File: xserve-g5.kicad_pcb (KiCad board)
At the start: 2 copper layers, 100 x 50 mm, 4 parts, among them J1 SATA_Backplane_PWR, J2 FAN_LEFT, J3 FAN_RIGHT, J4 PWR

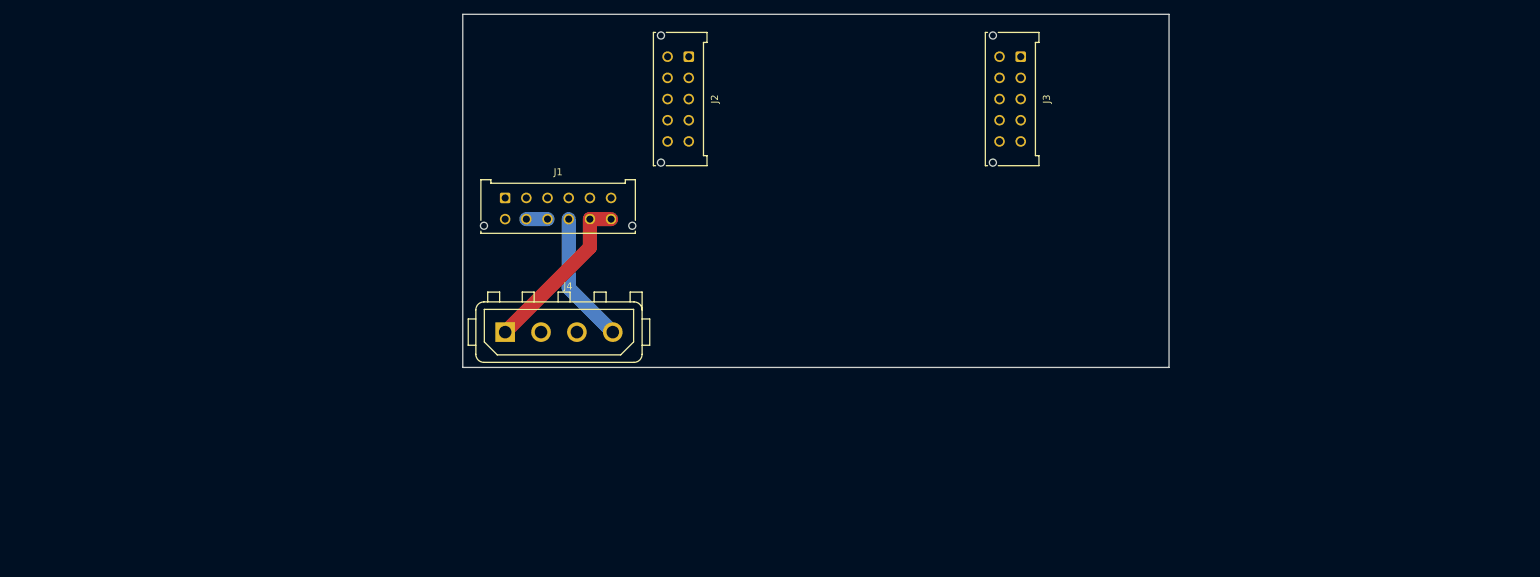
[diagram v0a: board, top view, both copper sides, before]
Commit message: update
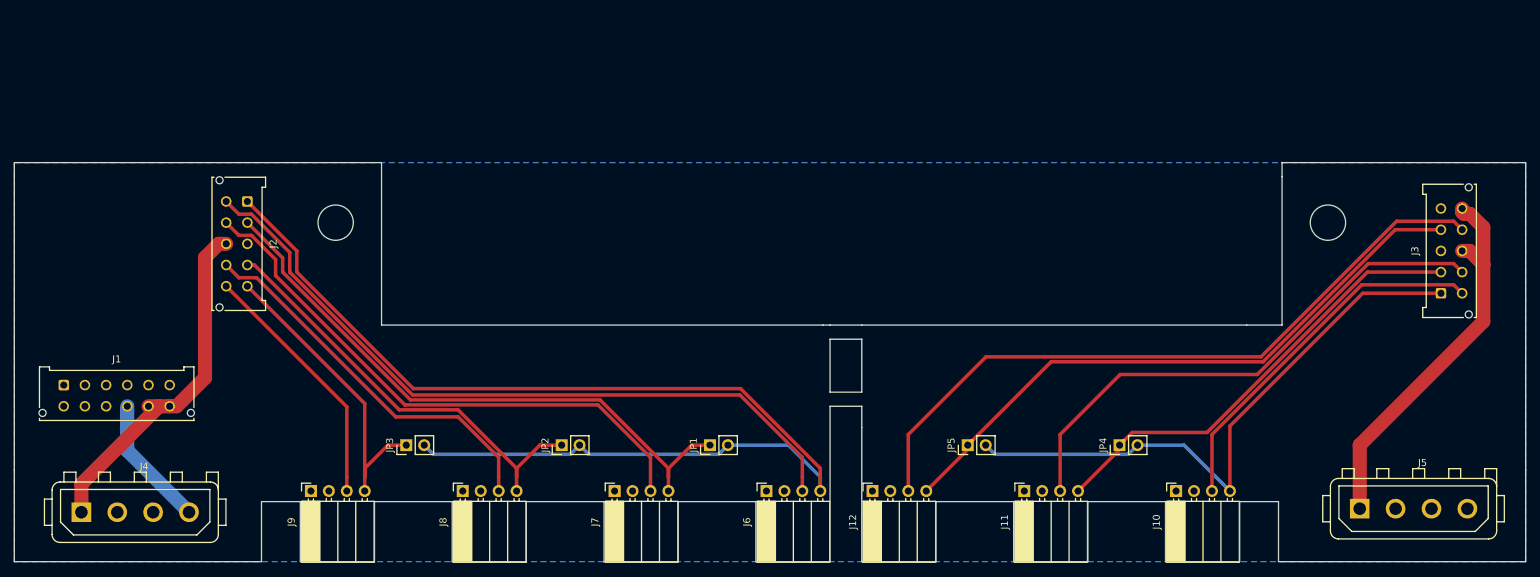
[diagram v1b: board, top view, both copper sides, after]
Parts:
- added J10: FAN5_PWM, Connector_PinSocket_2.54mm:PinSocket_1x04_P2.54mm_Horizontal, F.Cu at (191.0, 107.5)
- added J11: FAN6_PWM, Connector_PinSocket_2.54mm:PinSocket_1x04_P2.54mm_Horizontal, F.Cu at (169.5, 107.5)
- added J12: FAN7_PWM, Connector_PinSocket_2.54mm:PinSocket_1x04_P2.54mm_Horizontal, F.Cu at (148.0, 107.5)
- added J5: PWR_R, Connector_TE-Connectivity:TE_MATE-N-LOK_350211-1_1x04_P5.08mm_Vertical, F.Cu at (217.0, 110.0)
- added J6: FAN1_PWM, Connector_PinSocket_2.54mm:PinSocket_1x04_P2.54mm_Horizontal, F.Cu at (133.0, 107.5)
- added J7: FAN2_PWM, Connector_PinSocket_2.54mm:PinSocket_1x04_P2.54mm_Horizontal, F.Cu at (111.5, 107.5)
- added J8: FAN3_PWM, Connector_PinSocket_2.54mm:PinSocket_1x04_P2.54mm_Horizontal, F.Cu at (90.0, 107.5)
- added J9: FAN4_PWM, Connector_PinSocket_2.54mm:PinSocket_1x04_P2.54mm_Horizontal, F.Cu at (68.5, 107.5)
- added JP1: PWM1_2, Connector_PinHeader_2.54mm:PinHeader_1x02_P2.54mm_Vertical, F.Cu at (125.0, 101.0)
- added JP2: PWM1_3, Connector_PinHeader_2.54mm:PinHeader_1x02_P2.54mm_Vertical, F.Cu at (104.0, 101.0)
- added JP3: PWM1_4, Connector_PinHeader_2.54mm:PinHeader_1x02_P2.54mm_Vertical, F.Cu at (82.0, 101.0)
- added JP4: PWM5_6, Connector_PinHeader_2.54mm:PinHeader_1x02_P2.54mm_Vertical, F.Cu at (183.0, 101.0)
- added JP5: PWM5_7, Connector_PinHeader_2.54mm:PinHeader_1x02_P2.54mm_Vertical, F.Cu at (161.5, 101.0)
- J4: value PWR -> PWR_L
- moved J3 68.3 mm to (228.5, 79.5), turned to 90 degrees
- moved J1 67.9 mm to (33.5, 92.5)
- moved J2 65.8 mm to (59.5, 66.5)
- moved J4 65.2 mm to (36.0, 110.5)
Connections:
- J1 pad 8: +3V3 -> Net-(J1-Pad8)
- J1 pad 9: +3V3 -> Net-(J1-Pad9)
- J2 pad 1: Net-(J2-Pad1) -> PWM1
- J2 pad 10: Net-(J2-Pad10) -> TACH4
- J2 pad 2: Net-(J2-Pad2) -> PWM2
- J2 pad 3: Net-(J2-Pad3) -> GND
- J2 pad 4: Net-(J2-Pad4) -> PWM3
- J2 pad 5: Net-(J2-Pad5) -> PWM4
- J2 pad 6: Net-(J2-Pad6) -> TACH1
- J2 pad 7: Net-(J2-Pad7) -> TACH2
- J2 pad 8: Net-(J2-Pad8) -> +12V
- J2 pad 9: Net-(J2-Pad9) -> TACH3
- J3 pad 1: Net-(J3-Pad1) -> PWM5
- J3 pad 10: Net-(J3-Pad10) -> +12V
- J3 pad 2: Net-(J3-Pad2) -> PWM6
- J3 pad 3: Net-(J3-Pad3) -> GND
- J3 pad 4: Net-(J3-Pad4) -> PWM7
- J3 pad 5: Net-(J3-Pad5) -> GND
- J3 pad 6: Net-(J3-Pad6) -> TACH5
- J3 pad 7: Net-(J3-Pad7) -> TACH6
- J3 pad 8: Net-(J3-Pad8) -> +12V
- J3 pad 9: Net-(J3-Pad9) -> TACH7
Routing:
- net PWM1: track 0.00 -> 163.8 mm
- net TACH1: track 0.00 -> 103.0 mm
- net TACH7: track 0.00 -> 99.4 mm
- net PWM7: track 0.00 -> 88.6 mm
- net PWM2: track 0.00 -> 86.9 mm
- net PWM5: track 0.00 -> 85.2 mm
- net +12V: track 24.0 -> 105.3 mm
- net TACH2: track 0.00 -> 79.9 mm
- net TACH6: track 0.00 -> 75.4 mm
- net PWM6: track 0.00 -> 64.6 mm
- net PWM3: track 0.00 -> 62.2 mm
- net TACH3: track 0.00 -> 54.6 mm
- net TACH5: track 0.00 -> 52.7 mm
- net PWM4: track 0.00 -> 44.3 mm
- net TACH4: track 0.00 -> 36.1 mm
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- added copper zone on B.Cu, net GND
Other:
- board size 100 x 50 mm -> 214 x 56.5 mm
- net class GND added: clearance 0.2, trace_width 1, via_dia 0.8, via_drill 0.4
- net class PWM added: clearance 0.2, trace_width 0.5, via_dia 0.8, via_drill 0.4
- net class TACH added: clearance 0.2, trace_width 0.5, via_dia 0.8, via_drill 0.4
